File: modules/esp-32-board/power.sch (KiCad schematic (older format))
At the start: 11 parts, among them J5 Barrel_Jack_MountingPin, U2 NCP1117-3.3, U3 NCP1117ST50T3G

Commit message: Add custom symbols/footprints to project_components
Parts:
- J5: footprint Connector_BarrelJack:BarrelJack_CLIFF_FC68148_Horizontal -> project_components:BarrelJack_CLIFF_FC68148_Horizontal
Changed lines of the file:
@@
 F 0 "J5" H 1300 1400 50  0000 C CNN
 F 1 "Barrel_Jack_MountingPin" H 1500 1900 50  0000 C CNN
-F 2 "Connector_BarrelJack:BarrelJack_CLIFF_FC68148_Horizontal" H 1600 1610 50  0001 C CNN
+F 2 "project_components:BarrelJack_CLIFF_FC68148_Horizontal" H 1600 1610 50  0001 C CNN
 F 3 "https://www.tme.eu/Document/3d585bc2823a1d150d9d924b483e2fef/1613-21.pdf" H 1600 1610 50  0001 C CNN
 F 4 "tme.eu" H 1550 1650 50  0001 C CNN "Vendor"

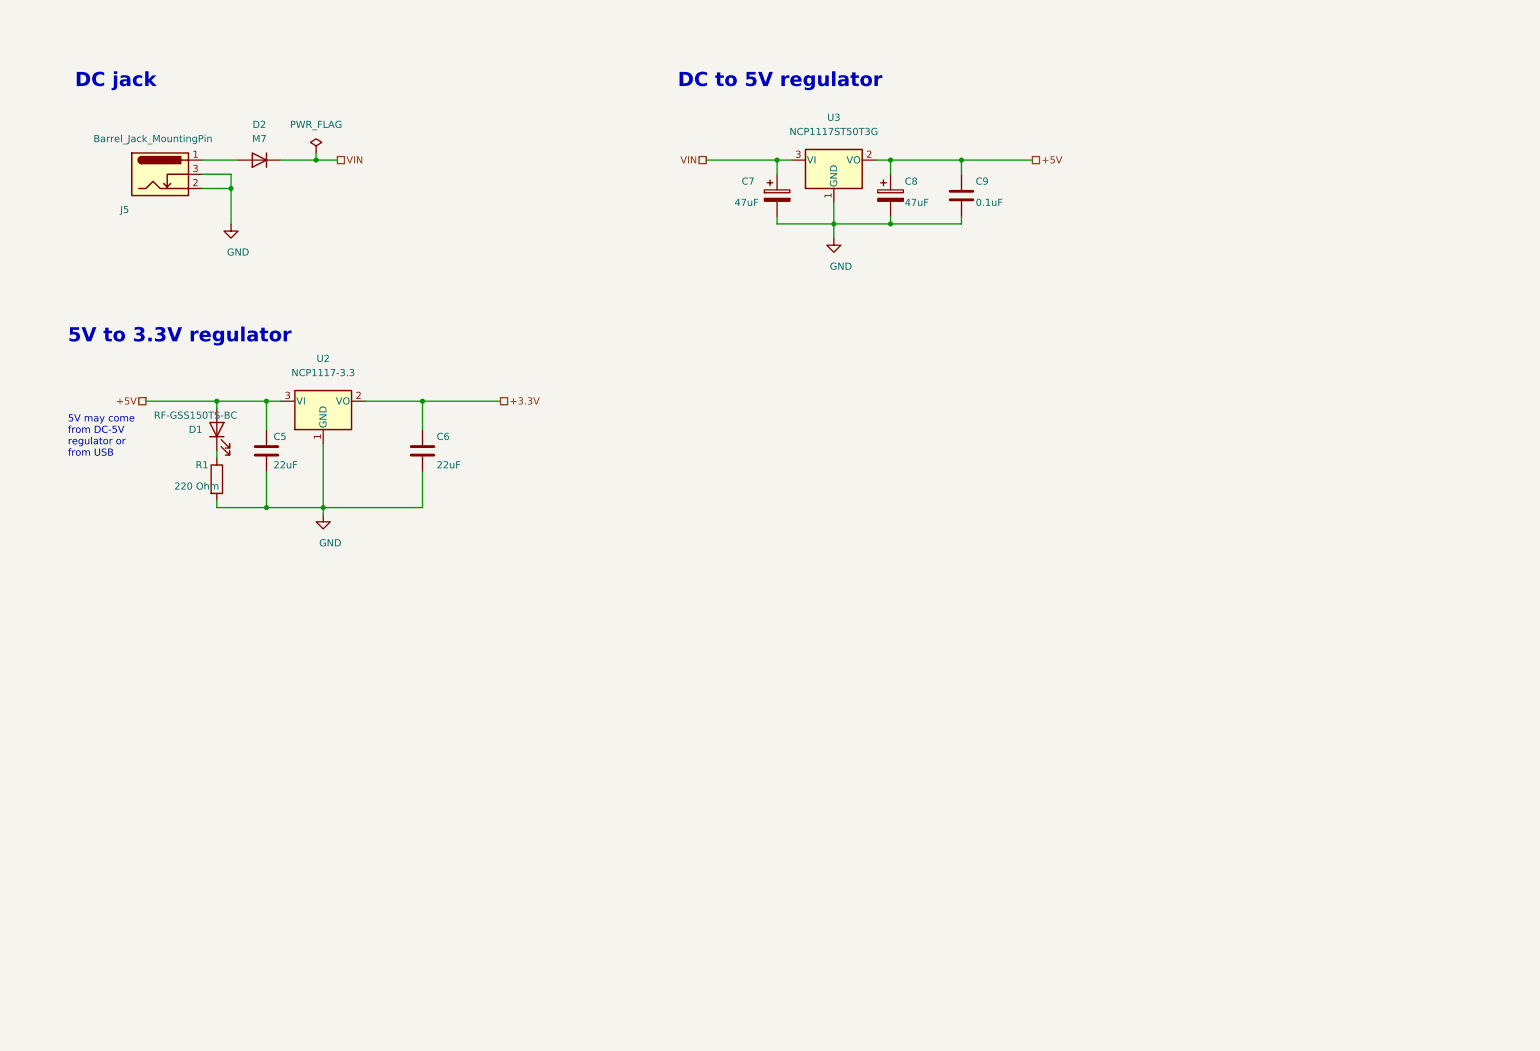
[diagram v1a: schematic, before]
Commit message: Documentational changes
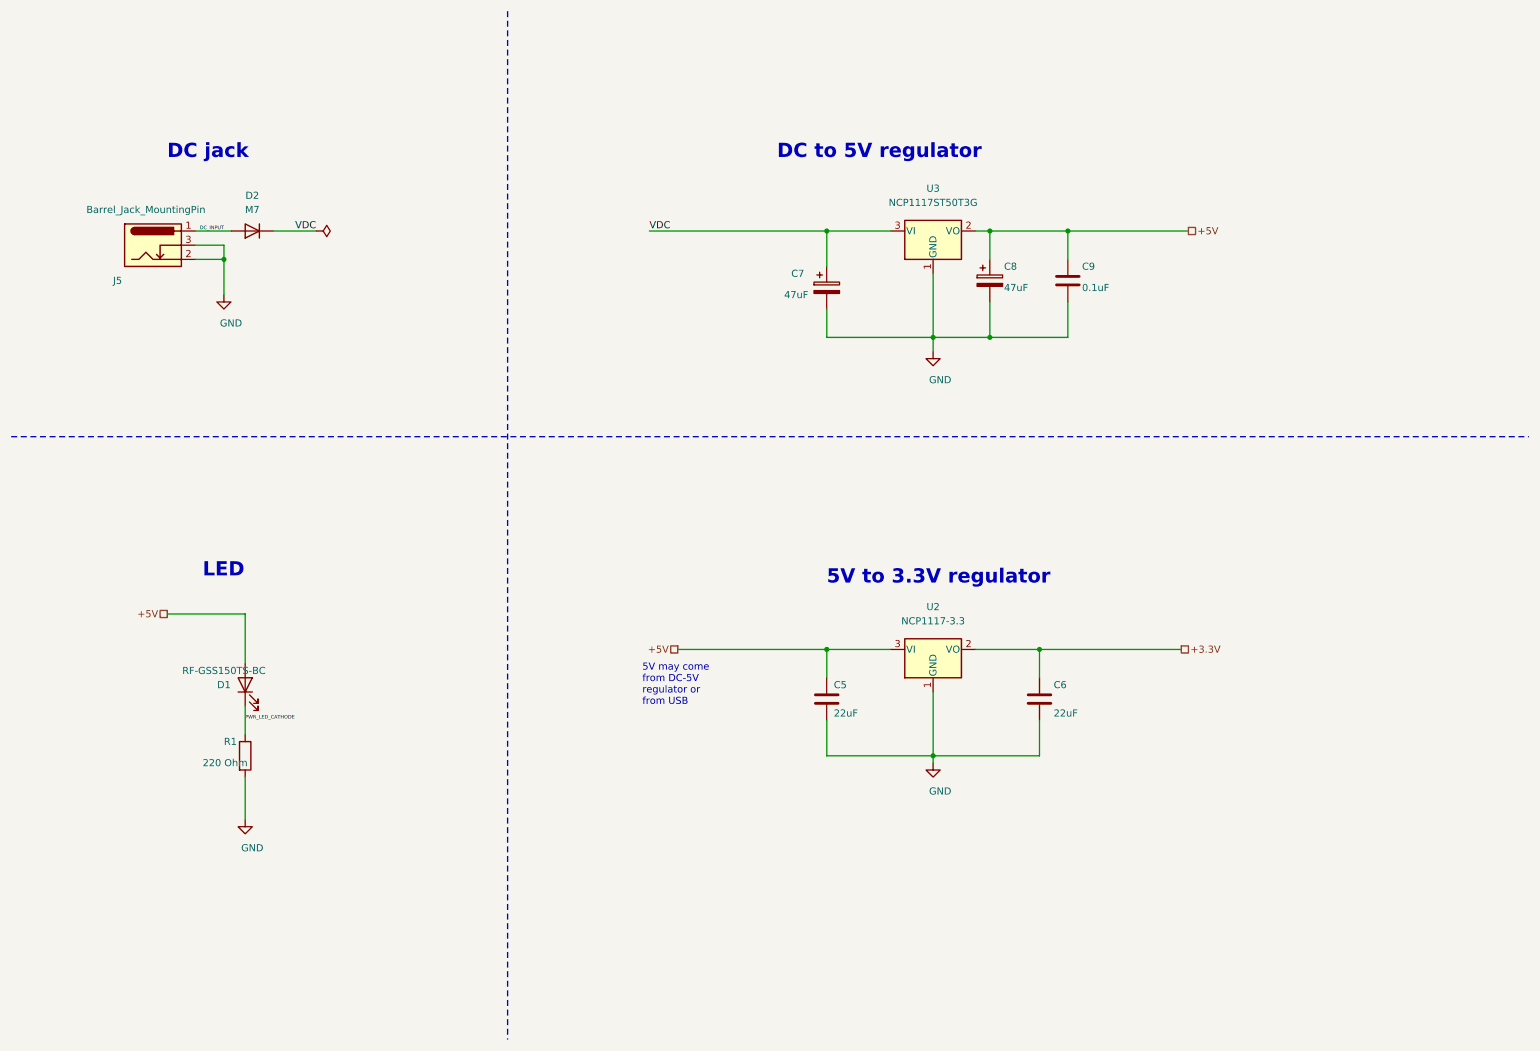
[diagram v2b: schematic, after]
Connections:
- net DC_INPUT: now reaches D2.2 (A), J5.1
- net PWR_LED_CATHODE: now reaches D1.1 (K), R1.1
- net VIN renamed VDC
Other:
- note added: "LED"
- moved on the sheet: C5, C6, C7, C8, C9, D1, D2, J5, R1, U2, U3
